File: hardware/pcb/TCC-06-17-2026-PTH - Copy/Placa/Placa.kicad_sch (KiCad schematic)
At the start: 81 parts, among them J1 Conn_01x03, J3 Conn_01x02, J6 Conn_01x03, J7 Conn_01x03, J8 Conn_01x02, SW1 SW_Push, SW10 SW_Push, SW11 SW_Push, SW12 SW_Push, SW13 SW_Push, SW14 SW_Push, SW15 SW_Push, SW16 SW_Push, SW17 SW_Push, SW18 SW_Push, SW19 SW_Push, SW2 SW_Push, SW20 SW_Push, SW21 SW_Push, SW22 SW_Push, SW23 SW_Push, SW24 SW_Push, SW25 SW_Push, SW26 SW_Push, SW27 SW_Push, SW28 SW_Push, SW29 SW_Push, SW3 SW_Push, SW30 SW_Push, SW31 SW_Push, SW32 SW_Push, SW33 SW_Push, SW34 SW_Push, SW35 SW_Push, SW36 SW_Push, SW37 SW_Push, SW38 SW_Push, SW4 SW_Push, SW5 SW_Push, SW6 SW_Push, SW7 SW_Push, SW8 SW_Push, SW9 SW_Push

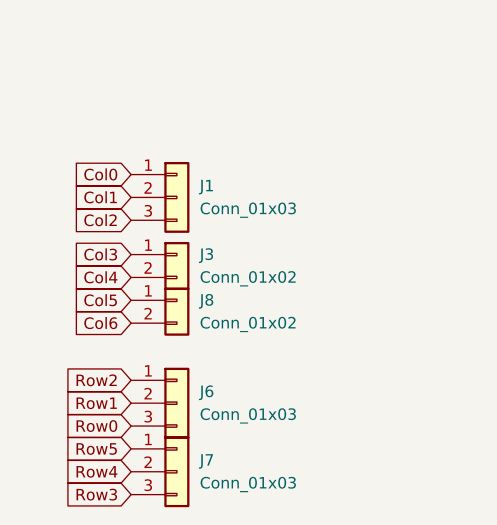
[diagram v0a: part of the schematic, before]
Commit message: Ajustes na pcb
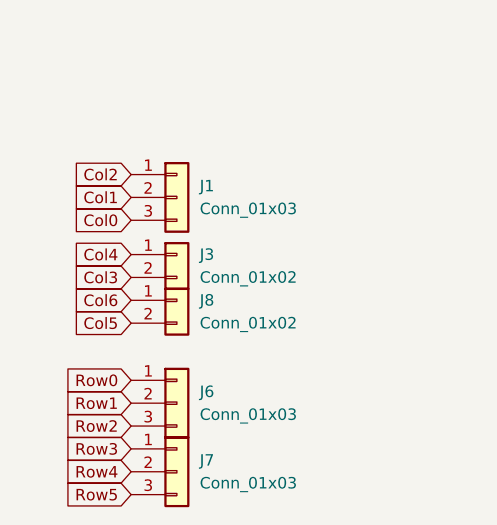
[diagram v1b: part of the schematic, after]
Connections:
- net Col0: now also J1.3 (Pin_3); no longer J1.1 (Pin_1)
- net Col2: now also J1.1 (Pin_1); no longer J1.3 (Pin_3)
- net Col3: now also J3.2 (Pin_2); no longer J3.1 (Pin_1)
- net Col4: now also J3.1 (Pin_1); no longer J3.2 (Pin_2)
- net Col5: now also J8.2 (Pin_2); no longer J8.1 (Pin_1)
- net Col6: now also J8.1 (Pin_1); no longer J8.2 (Pin_2)
- net Row0: now also J6.1 (Pin_1); no longer J6.3 (Pin_3)
- net Row2: now also J6.3 (Pin_3); no longer J6.1 (Pin_1)
- net Row3: now also J7.1 (Pin_1); no longer J7.3 (Pin_3)
- net Row5: now also J7.3 (Pin_3); no longer J7.1 (Pin_1)
